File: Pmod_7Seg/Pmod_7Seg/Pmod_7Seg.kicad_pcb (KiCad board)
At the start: 2 copper layers, 68.5 x 42.4 mm, 14 parts, among them IC1 TBD62783APG, IC2 TBD62003APG, IC3 OSL60362-LR, J1 Conn_02x06_Counter_Clockwise, J2 Conn_02x06_Counter_Clockwise

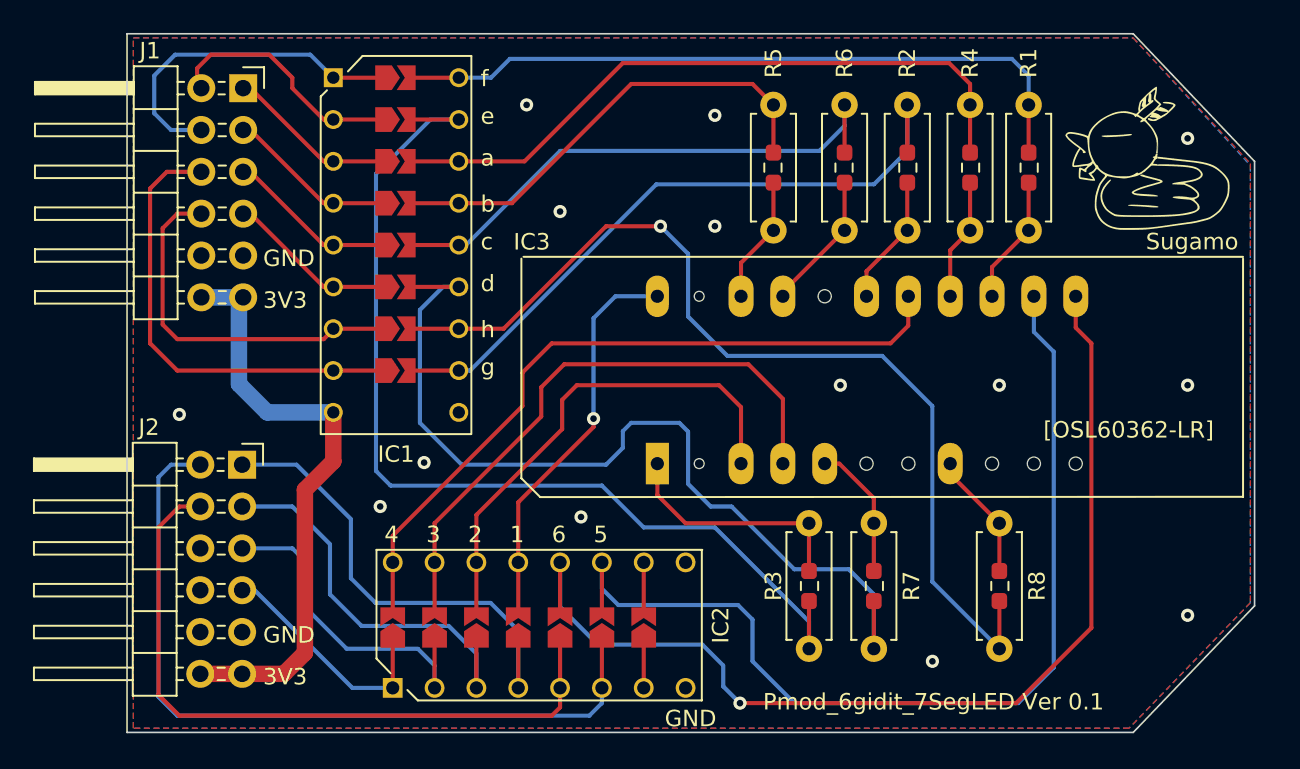
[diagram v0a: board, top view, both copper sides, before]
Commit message: 0830
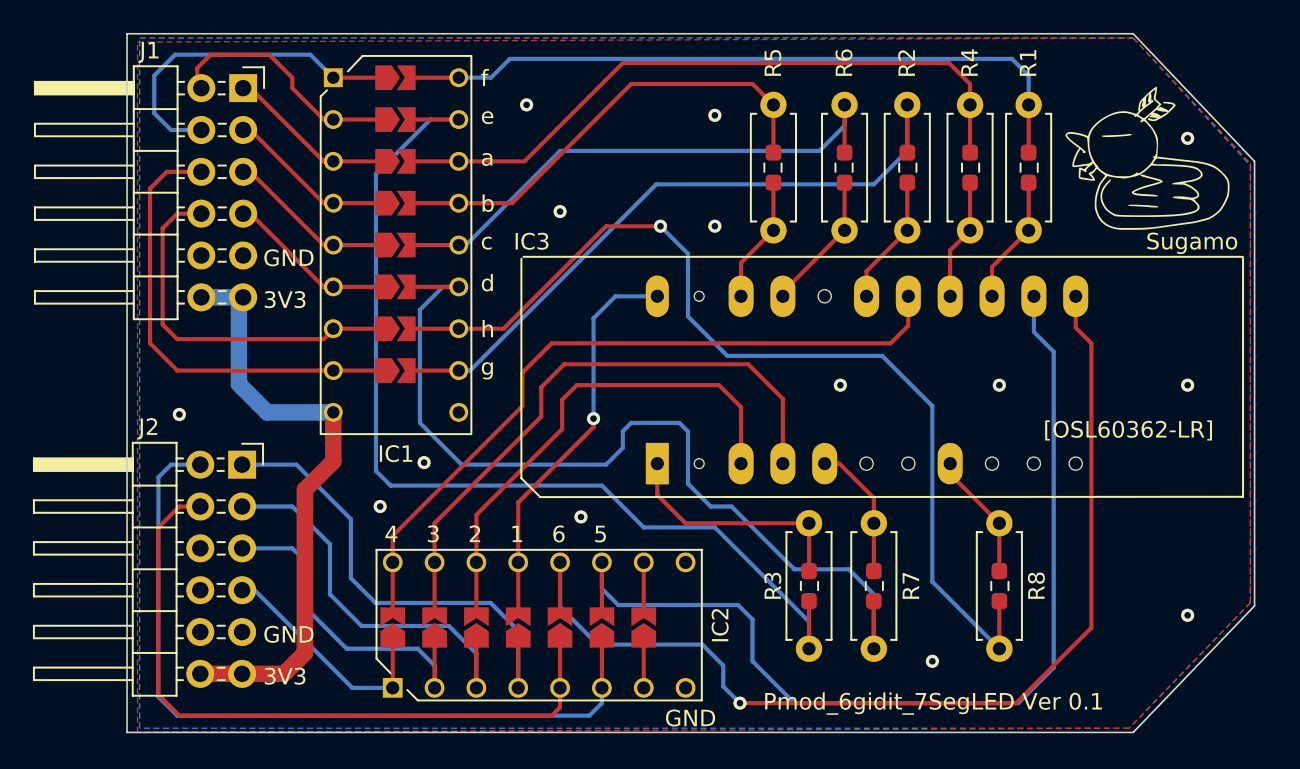
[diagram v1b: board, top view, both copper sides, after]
